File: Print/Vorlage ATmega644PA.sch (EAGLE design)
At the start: 56 parts, among them IC1 ATmega644PA, IC4 ATTINY24/44/84-SSU, Q1 16MHz, X3 87758-3416

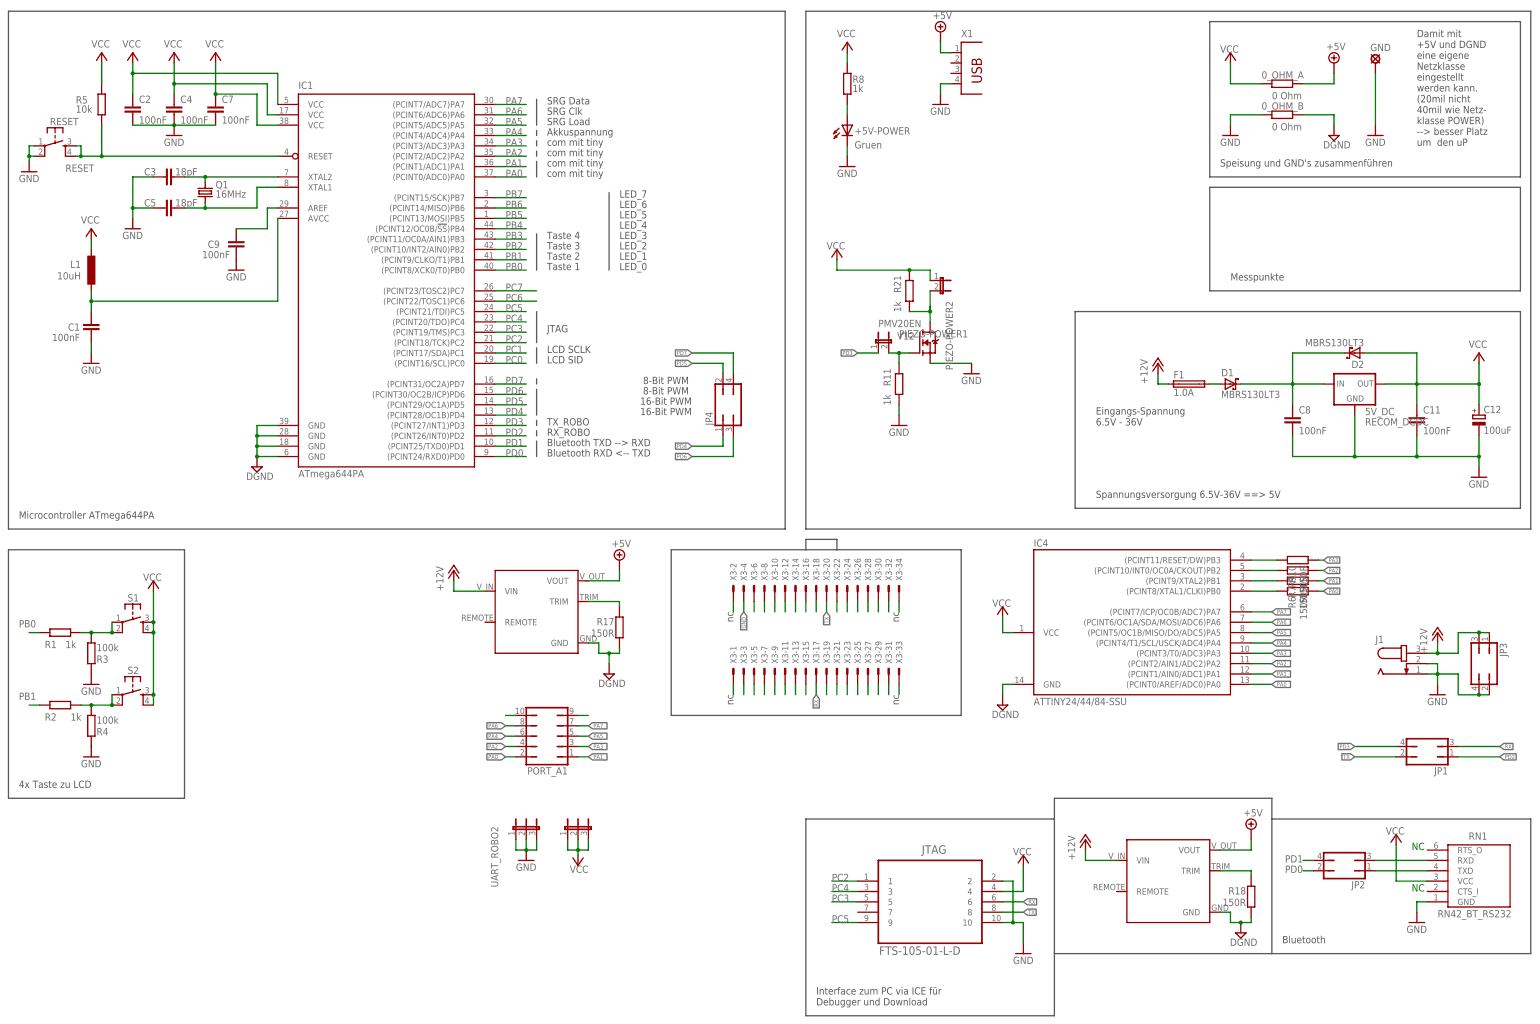
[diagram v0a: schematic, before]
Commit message: sf
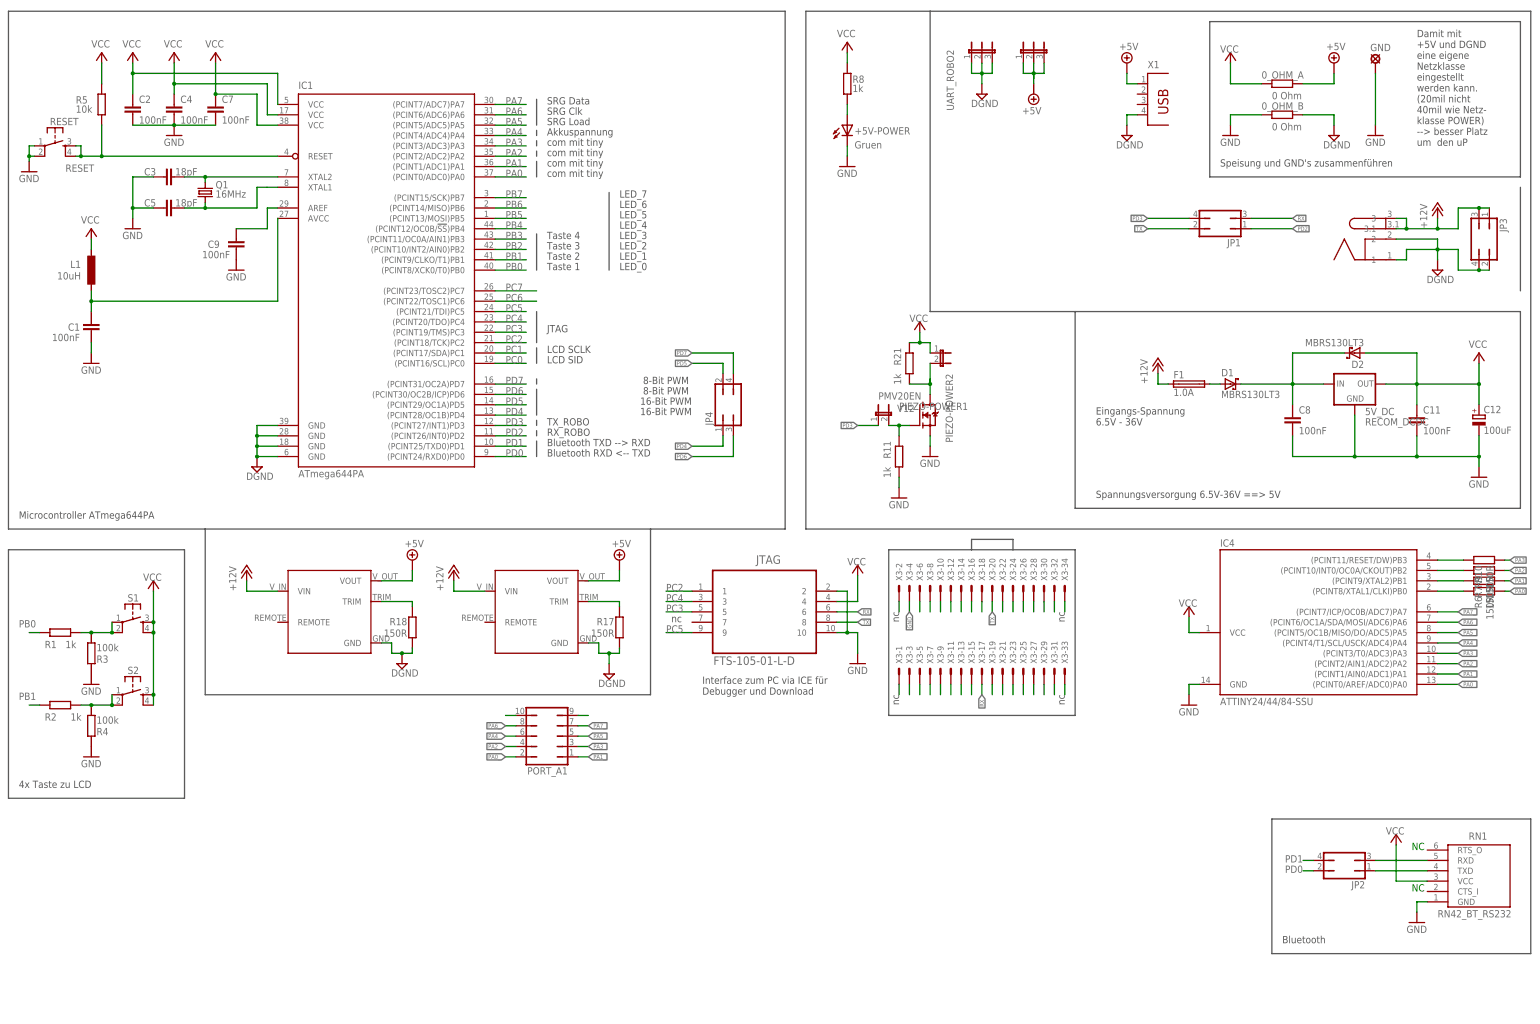
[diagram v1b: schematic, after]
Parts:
- removed J1: (no value), con-jack:JACK-PLUG0
- added U$1: BUCHSE, untitled:BUCHSE
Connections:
- net +12V: now also U$1.3, U$1.3.1; no longer J1.3
- net +5V: now also UART_ROBO1.1, UART_ROBO1.2, UART_ROBO1.3
- net DGND: now also JP3.2, JP3.4, U$1.1, U$1.2, UART_ROBO2.1, UART_ROBO2.2, UART_ROBO2.3, X1.4; no longer IC4.GND
- net GND: now also IC4.GND; no longer J1.1, J1.2, JP3.2, JP3.4, UART_ROBO2.1, UART_ROBO2.2, UART_ROBO2.3, X1.4
- net VCC: no longer UART_ROBO1.1, UART_ROBO1.2, UART_ROBO1.3
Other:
- note removed: "Messpunkte"
- moved on the sheet: IC4, JP1, JP3, JTAG, PIEZO-POWER1, PIEZO-POWER2, R10, R11, R18, R21, R6, R7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
